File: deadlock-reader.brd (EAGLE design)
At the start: 49.2 x 49.5 mm, 49 parts, among them IC1 LM386M-1, IC2 STM32F072XX, IC3 MCP16301/H, IC4 MAX3232CSE, J1 RJ12 6p6c, X1 MINI-USB-SCHIELD-32005-301

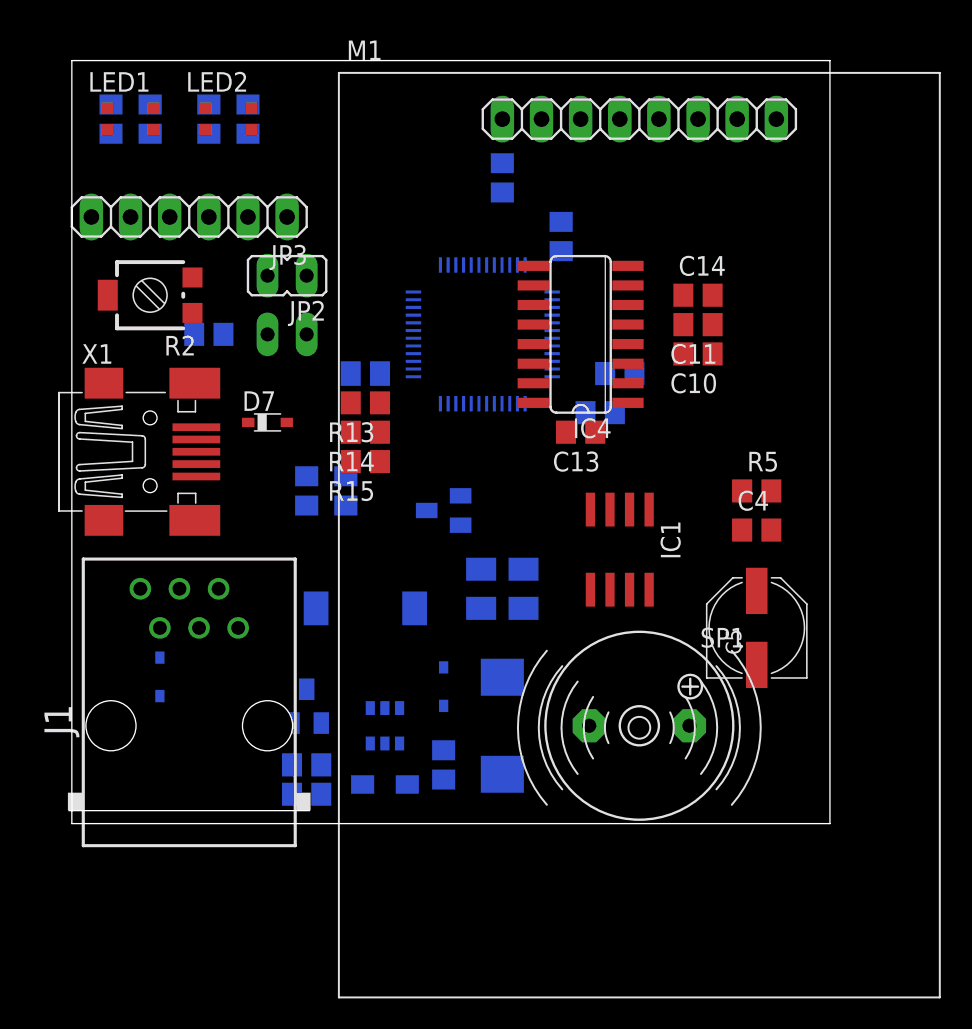
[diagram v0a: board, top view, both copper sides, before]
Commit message: Optimize component placements
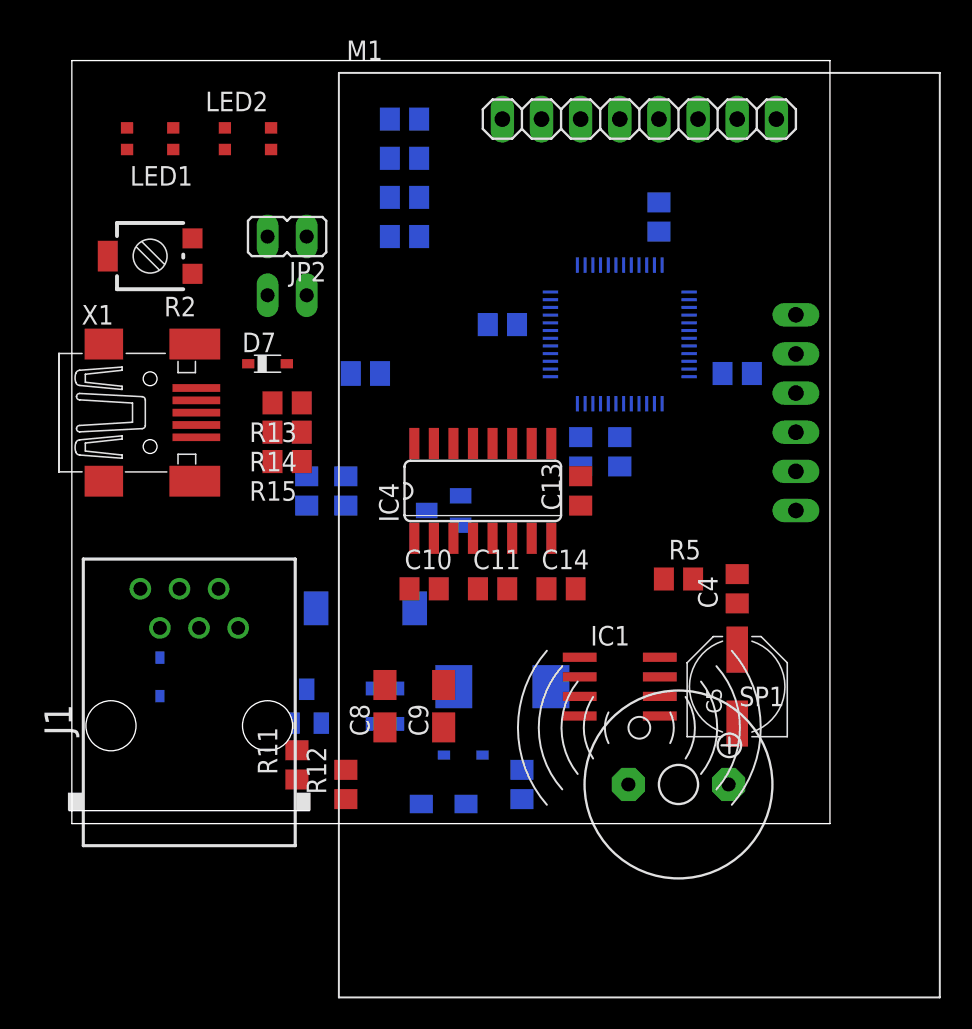
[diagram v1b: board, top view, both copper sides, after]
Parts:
- moved JP3 41.4 mm to (47.0, 26.7), flipped to the bottom, turned to 270 degrees
- moved R6 27.7 mm to (35.6, 24.1), turned to 90 degrees
- moved C10 23.4 mm to (22.9, 15.2), turned to 0 degrees
- moved C11 21.7 mm to (27.3, 15.2), turned to 0 degrees
- moved C14 21.0 mm to (31.8, 15.2)
- moved C12 19.8 mm to (43.2, 29.2), turned to 180 degrees
- moved R7 19.1 mm to (21.6, 45.7), turned to 180 degrees
- moved R8 18.2 mm to (21.6, 38.1), turned to 180 degrees
- moved R9 13.7 mm to (21.6, 40.6), turned to 180 degrees
- moved IC4 12.0 mm to (26.7, 21.6), turned to 0 degrees
- moved R10 10.5 mm to (21.6, 43.2), turned to 180 degrees
- moved C8 9.92 mm to (20.3, 7.62), flipped to the top, turned to 90 degrees
- moved C9 9.67 mm to (24.1, 7.62), flipped to the top, turned to 90 degrees
- moved IC1 8.89 mm to (35.6, 8.89), turned to 270 degrees
- moved IC2 8.89 mm to (35.6, 31.8), turned to 90 degrees
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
